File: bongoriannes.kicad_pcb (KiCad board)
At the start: 2 copper layers, 100 x 80 mm, 74 parts, among them J1 VRAM, J10 VIDEO, J11 PPU21, J13 SOUND, J14 POWER, J2 CART_FRONT, J3 CART_BOTTOM, J4 CPU_RP2A03, J5 PRG_WRAM, J7 PPU, P1 P1, P2 P2, Q1 2SC2021, Q2 2SC2021, Q3 2SA937, SW1 SW_Push, U1 74LS373, U2 74LS139, U3 74LS368, U4 74LS368, Y1 21.47727

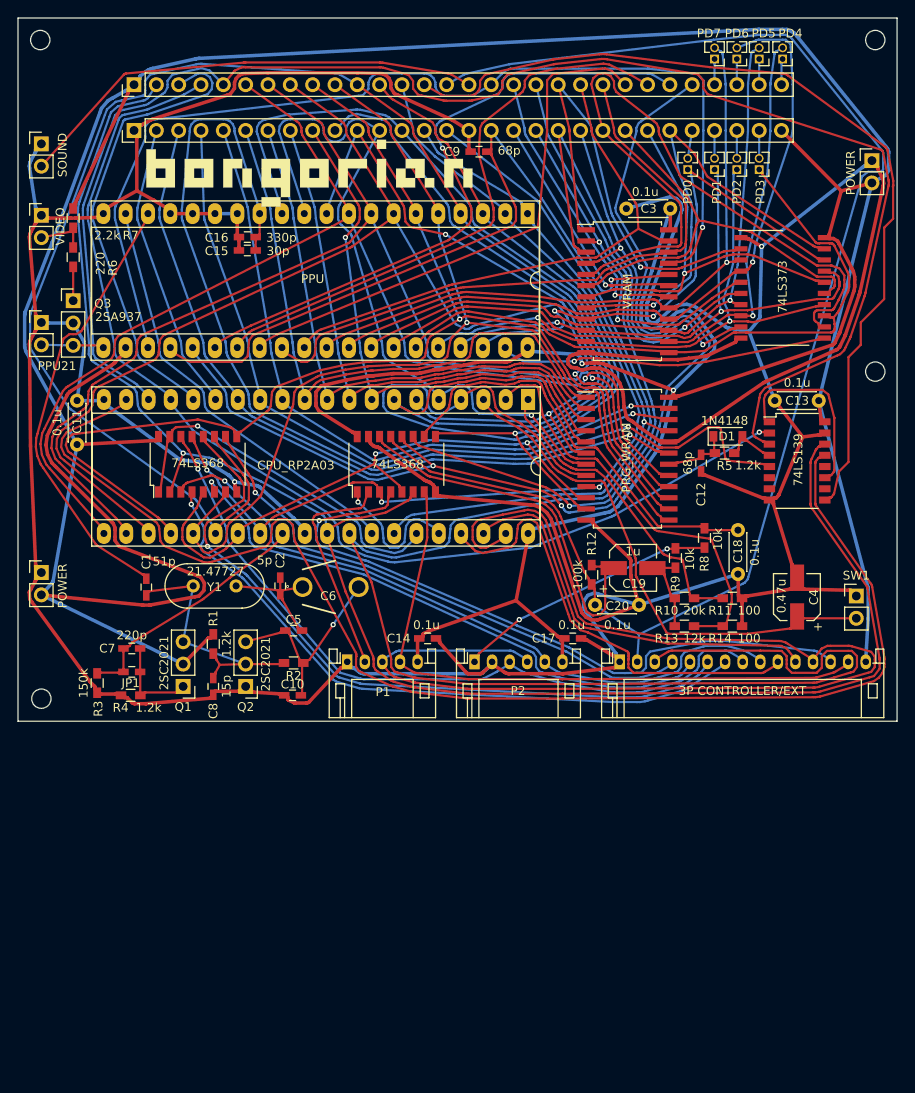
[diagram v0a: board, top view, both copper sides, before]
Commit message: meishi_size
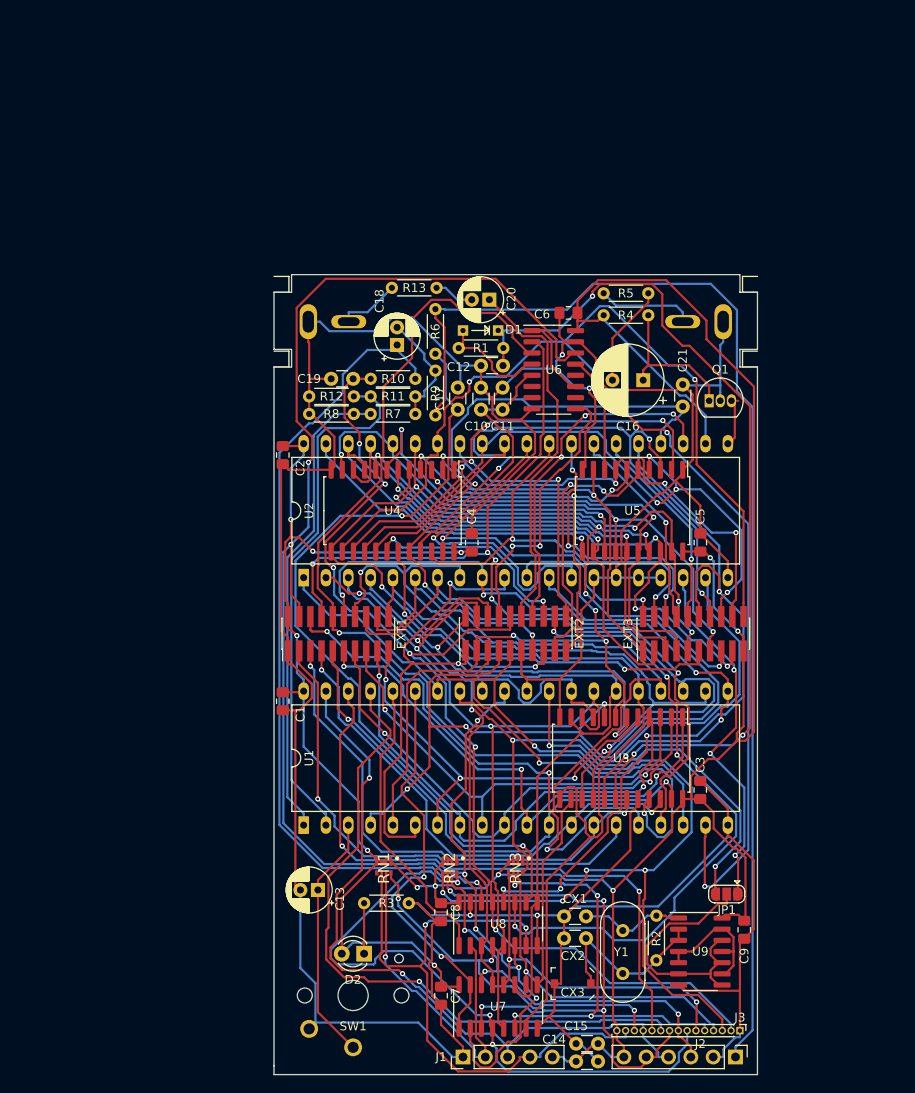
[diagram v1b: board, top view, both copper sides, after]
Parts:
- removed 3P CONTROLLER/EXT: EXT, Connectors_JST:JST_PH_S15B-PH-K_15x2.00mm_Angled
- removed G*** (x2): LOGO, GAME:bongorian
- removed G***: LOGO, GAME:fami
- removed J10: VIDEO, Pin_Headers:Pin_Header_Straight_1x02_Pitch2.54mm
- removed J11: PPU21, Pin_Headers:Pin_Header_Straight_1x02_Pitch2.54mm
- removed J13: SOUND, Pin_Headers:Pin_Header_Straight_1x02_Pitch2.54mm
- removed J14: POWER, Pin_Headers:Pin_Header_Straight_1x02_Pitch2.54mm
- removed J7: PPU, Housings_DIP:DIP-40_W15.24mm_Socket_LongPads
- removed JP15: PD0, Pin_Headers:Pin_Header_Straight_1x02_Pitch1.27mm
- removed JP17: PD1, Pin_Headers:Pin_Header_Straight_1x02_Pitch1.27mm
- removed JP18: PD7, Pin_Headers:Pin_Header_Straight_1x02_Pitch1.27mm
- removed JP19: PD2, Pin_Headers:Pin_Header_Straight_1x02_Pitch1.27mm
- removed JP20: PD6, Pin_Headers:Pin_Header_Straight_1x02_Pitch1.27mm
- removed JP21: PD3, Pin_Headers:Pin_Header_Straight_1x02_Pitch1.27mm
- removed JP22: PD5, Pin_Headers:Pin_Header_Straight_1x02_Pitch1.27mm
- removed JP23: PD4, Pin_Headers:Pin_Header_Straight_1x02_Pitch1.27mm
- removed P1: P1, Connectors_JST:JST_PH_S5B-PH-K_05x2.00mm_Angled
- removed P2: P2, Connectors_JST:JST_PH_S6B-PH-K_06x2.00mm_Angled
- removed POWER: Conn_01x02, Pin_Headers:Pin_Header_Straight_1x02_Pitch2.54mm
- removed Q2: 2SC2021, Pin_Headers:Pin_Header_Straight_1x03_Pitch2.54mm
- removed Q3: 2SA937, Pin_Headers:Pin_Header_Straight_1x03_Pitch2.54mm
- removed R14: 100, Resistors_SMD:R_0603_HandSoldering
- removed hole1, hole2, hole3, hole4: MountingHole_2.2mm_M2, Mounting_Holes:MountingHole_2.2mm_M2
- added C21: 68p, Capacitor_THT:C_Disc_D3.0mm_W1.6mm_P2.50mm, F.Cu at (146.5, 85.0)
- added CX1: 22p, Capacitor_THT:C_Disc_D3.0mm_W1.6mm_P2.50mm, F.Cu at (135.5, 143.0)
- added CX2: 15p, Capacitor_THT:C_Disc_D3.0mm_W1.6mm_P2.50mm, F.Cu at (135.5, 145.5)
- added CX3: CTRIM, Capacitor_SMD:C_Trimmer_Murata_TZC3, F.Cu at (134.0, 150.7)
- added D2: LED, LED_THT:LED_D3.0mm, F.Cu at (110.2, 147.2)
- added EXT1: 1-10, Connector_PinHeader_1.27mm:PinHeader_2x10_P1.27mm_Vertical_SMD, F.Cu at (107.3, 110.8)
- added EXT2: 11-20, Connector_PinHeader_1.27mm:PinHeader_2x10_P1.27mm_Vertical_SMD, F.Cu at (127.5, 110.8)
- added EXT3: 21-30, Connector_PinHeader_1.27mm:PinHeader_2x10_P1.27mm_Vertical_SMD, F.Cu at (147.7, 110.8)
- added RN1: MNR04MRAPJ103, bongorian:RESCAX50P100X200X36-8N, F.Cu at (112.5, 137.5)
- added RN2: MNR04MRAPJ103, bongorian:RESCAX50P100X200X36-8N, F.Cu at (120.0, 137.5)
- added RN3: MNR04MRAPJ103, bongorian:RESCAX50P100X200X36-8N, F.Cu at (127.5, 137.5)
- added U5: 74LS373, Package_SO:SOIC-20W_7.5x12.8mm_P1.27mm, F.Cu at (140.8, 96.8)
- added U6: 74LS139, Package_SO:SOIC-16_3.9x9.9mm_P1.27mm, F.Cu at (131.8, 80.8)
- added U7: 74LS368, Package_SO:SOIC-16_3.9x9.9mm_P1.27mm, F.Cu at (125.5, 153.2)
- added U8: 74LS368, Package_SO:SOIC-16_3.9x9.9mm_P1.27mm, F.Cu at (125.5, 143.9)
- added U9: 74HC04, Package_SO:SOIC-14_3.9x8.7mm_P1.27mm, F.Cu at (148.5, 147.0)
- C1: value 51p -> 0.1u; footprint Capacitors_SMD:C_0603_HandSoldering -> Capacitor_SMD:C_0805_2012Metric_Pad1.15x1.40mm_HandSolder
- C10: value 51p -> 330p; footprint Capacitors_SMD:C_0603_HandSoldering -> Capacitor_THT:C_Disc_D3.0mm_W1.6mm_P2.50mm
- C11: value 0.1u -> 30p; footprint Capacitors_THT:C_Disc_D4.3mm_W1.9mm_P5.00mm -> Capacitor_THT:C_Disc_D3.0mm_W1.6mm_P2.50mm
- C12, C14, C17: footprint Capacitors_SMD:C_0603_HandSoldering -> Capacitor_THT:C_Disc_D3.0mm_W1.6mm_P2.50mm
- C13: value 0.1u -> 0.47u; footprint Capacitors_THT:C_Disc_D4.3mm_W1.9mm_P5.00mm -> Capacitor_THT:CP_Radial_D5.0mm_P2.00mm
- C15: value 30p -> 0.1u; footprint Capacitors_SMD:C_0603_HandSoldering -> Capacitor_THT:C_Disc_D3.0mm_W1.6mm_P2.50mm
- C16: value 330p -> 220u; footprint Capacitors_SMD:C_0603_HandSoldering -> Capacitor_THT:CP_Radial_D8.0mm_P3.50mm
- C18: value 0.1u -> 1u; footprint Capacitors_THT:C_Disc_D4.3mm_W1.9mm_P5.00mm -> Capacitor_THT:CP_Radial_D5.0mm_P2.00mm
- C19: value 1u -> 0.1u; footprint Capacitors_SMD:CP_Elec_5x5.3 -> Capacitor_THT:C_Disc_D3.0mm_W1.6mm_P2.50mm
- C2: value 5p -> 0.1u; footprint Capacitors_SMD:C_0603_HandSoldering -> Capacitor_SMD:C_0805_2012Metric_Pad1.15x1.40mm_HandSolder
- C20: value 0.1u -> 4.7u; footprint Capacitors_THT:C_Disc_D4.3mm_W1.9mm_P5.00mm -> Capacitor_THT:CP_Radial_D5.0mm_P2.00mm
- C3: footprint Capacitors_THT:C_Disc_D4.3mm_W1.9mm_P5.00mm -> Capacitor_SMD:C_0805_2012Metric_Pad1.15x1.40mm_HandSolder
- C4: value 0.47u -> 0.1u; footprint Capacitors_SMD:CP_Elec_5x5.3 -> Capacitor_SMD:C_0805_2012Metric_Pad1.15x1.40mm_HandSolder
- C5: value 18p -> 0.1u; footprint Capacitors_SMD:C_0603_HandSoldering -> Capacitor_SMD:C_0805_2012Metric_Pad1.15x1.40mm_HandSolder
- C6: value 30p -> 0.1u; footprint SamacSys_Parts:TZ03(B) -> Capacitor_SMD:C_0805_2012Metric_Pad1.15x1.40mm_HandSolder
- C7: value 220p -> 0.1u; footprint Capacitors_SMD:C_0603_HandSoldering -> Capacitor_SMD:C_0805_2012Metric_Pad1.15x1.40mm_HandSolder
- C8: value 15p -> 0.1u; footprint Capacitors_SMD:C_0603_HandSoldering -> Capacitor_SMD:C_0805_2012Metric_Pad1.15x1.40mm_HandSolder
- C9: value 68p -> 0.1u; footprint Capacitors_SMD:C_0603_HandSoldering -> Capacitor_SMD:C_0805_2012Metric_Pad1.15x1.40mm_HandSolder
- D1: value 1N4148 -> 1S953; footprint Diodes_SMD:D_SOD-123 -> bongorian:DIODE_SHORT
- J1: value VRAM -> P1; footprint Housings_SOIC:SOIC-24W_7.5x15.4mm_Pitch1.27mm -> Connector_PinHeader_2.54mm:PinHeader_1x05_P2.54mm_Vertical
- J2: value CART_FRONT -> P2; footprint Pin_Headers:Pin_Header_Straight_1x30_Pitch2.54mm -> Connector_PinHeader_2.54mm:PinHeader_1x06_P2.54mm_Vertical
- J3: value CART_BOTTOM -> P3; footprint Pin_Headers:Pin_Header_Straight_1x30_Pitch2.54mm -> Connector_PinHeader_1.00mm:PinHeader_1x15_P1.00mm_Vertical
- J4: value CPU_RP2A03 -> VIDEO; footprint Housings_DIP:DIP-40_W15.24mm_Socket_LongPads -> bongorian:RCA_RJ2410N
- J5: value PRG_WRAM -> AUDIO; footprint Housings_SOIC:SOIC-24W_7.5x15.4mm_Pitch1.27mm -> bongorian:RCA_RJ2410N
- JP1: value Jumper -> CLOCK; footprint Capacitors_SMD:C_0603_HandSoldering -> Jumper:SolderJumper-3_P1.3mm_Open_RoundedPad1.0x1.5mm
- Q1: value 2SC2021 -> 2SA1015; footprint Pin_Headers:Pin_Header_Straight_1x03_Pitch2.54mm -> Package_TO_SOT_THT:TO-92_Inline
- R1, R9: footprint Resistors_SMD:R_0603_HandSoldering -> Resistor_THT:R_Axial_DIN0204_L3.6mm_D1.6mm_P5.08mm_Horizontal
- R10: value 20k -> 100k; footprint Resistors_SMD:R_0603_HandSoldering -> Resistor_THT:R_Axial_DIN0204_L3.6mm_D1.6mm_P5.08mm_Horizontal
- R11: value 100 -> 12k; footprint Resistors_SMD:R_0603_HandSoldering -> Resistor_THT:R_Axial_DIN0204_L3.6mm_D1.6mm_P5.08mm_Horizontal
- R12: value 100k -> 100; footprint Resistors_SMD:R_0603_HandSoldering -> Resistor_THT:R_Axial_DIN0204_L3.6mm_D1.6mm_P5.08mm_Horizontal
- R13: value 12k -> 1k; footprint Resistors_SMD:R_0603_HandSoldering -> Resistor_THT:R_Axial_DIN0204_L3.6mm_D1.6mm_P5.08mm_Horizontal
- R2: value 220k -> 1M; footprint Resistors_SMD:R_0603_HandSoldering -> Resistor_THT:R_Axial_DIN0204_L3.6mm_D1.6mm_P5.08mm_Horizontal
- R3: value 150k -> R; footprint Resistors_SMD:R_0603_HandSoldering -> Resistor_THT:R_Axial_DIN0204_L3.6mm_D1.6mm_P5.08mm_Horizontal
- R4: value 1.2k -> 150; footprint Resistors_SMD:R_0603_HandSoldering -> Resistor_THT:R_Axial_DIN0204_L3.6mm_D1.6mm_P5.08mm_Horizontal
- R5: value 1.2k -> 75; footprint Resistors_SMD:R_0603_HandSoldering -> Resistor_THT:R_Axial_DIN0204_L3.6mm_D1.6mm_P5.08mm_Horizontal
- R6: value 220 -> 10k; footprint Resistors_SMD:R_0603_HandSoldering -> Resistor_THT:R_Axial_DIN0204_L3.6mm_D1.6mm_P5.08mm_Horizontal
- R7: value 2.2k -> 20k; footprint Resistors_SMD:R_0603_HandSoldering -> Resistor_THT:R_Axial_DIN0204_L3.6mm_D1.6mm_P5.08mm_Horizontal
- R8: value 10k -> 100; footprint Resistors_SMD:R_0603_HandSoldering -> Resistor_THT:R_Axial_DIN0204_L3.6mm_D1.6mm_P5.08mm_Horizontal
- SW1: footprint Pin_Headers:Pin_Header_Straight_1x02_Pitch2.54mm -> keyswitches:PG1350
- U1: value 74LS373 -> 2A03_CPU; footprint Housings_SOIC:SO-20_12.8x7.5mm_Pitch1.27mm -> bongorian:DIP-40_W15.24mm_LongPads_hoso
- U2: value 74LS139 -> 2C02_PPU; footprint Housings_SSOP:SOP-16_4.4x10.4mm_Pitch1.27mm -> bongorian:DIP-40_W15.24mm_LongPads_hoso
- U3: value 74LS368 -> SRAM; footprint Housings_SSOP:SOP-16_4.4x10.4mm_Pitch1.27mm -> Package_SO:SOIC-24W_7.5x15.4mm_P1.27mm
- U4: value 74LS368 -> VRAM; footprint Housings_SSOP:SOP-16_4.4x10.4mm_Pitch1.27mm -> Package_SO:SOIC-24W_7.5x15.4mm_P1.27mm
- Y1: value 21.47727 -> Crystal; footprint Crystals:Crystal_HC49-U_Vertical -> Crystal:Crystal_HC49-4H_Vertical
- moved J3 127.8 mm to (153.0, 156.0), turned to 270 degrees
- moved J2 125.7 mm to (152.5, 159.0), turned to 270 degrees
- moved C15 97.7 mm to (134.4, 157.5)
- moved C9 93.5 mm to (153.5, 144.5), turned to 270 degrees
- moved J1 89.1 mm to (121.5, 159.0), turned to 90 degrees
- moved C13 76.2 mm to (105.0, 140.0), turned to 180 degrees
- moved SW1 73.1 mm to (109.0, 152.0)
- moved JP1 72.2 mm to (151.5, 140.5), turned to 180 degrees
- moved R4 69.0 mm to (137.5, 74.6), turned to 0 degrees
- moved Q1 68.1 mm to (149.5, 84.3), turned to 0 degrees
- moved C3 66.7 mm to (148.5, 128.6), turned to 90 degrees
- moved Y1 62.7 mm to (139.7, 144.6), turned to 270 degrees
- moved U1 61.5 mm to (127.5, 125.0), turned to 90 degrees
- moved U3 58.6 mm to (139.5, 125.0), turned to 270 degrees
- moved R2 53.4 mm to (143.5, 148.0), turned to 90 degrees
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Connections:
- C1 pad 1: PPU_CLK -> VCC
- C1 pad 2: Net-(C1-Pad2) -> GND
- C10 pad 1: GND -> /DBE#
- C10 pad 2: Net-(C10-Pad2) -> GND
- C11 pad 1: GND -> /DBE#
- C11 pad 2: VCC -> GND
- C13 pad 1: GND -> /RES#$%
- C13 pad 2: VCC -> GND
- C14 pad 1: VCC -> GND
- C14 pad 2: GND -> VCC
- C15 pad 2: DBE# -> VCC
- C16 pad 1: GND -> Net-(C16-Pad1)
- C16 pad 2: DBE# -> Net-(C16-Pad2)
- C17 pad 1: VCC -> /MIC_IN'
- C18 pad 1: MICIN' -> /SOUND_I'
- C18 pad 2: GND -> Net-(C18-Pad2)
- C19 pad 1: SOUNDI' -> /SOUND_I
- C19 pad 2: Net-(C19-Pad2) -> GND
- C2 pad 1: Net-(C2-Pad1) -> VCC
- C2 pad 2: Net-(C2-Pad1) -> GND
- C20 pad 1: SOUNDI -> /SOUND_OUT
- C20 pad 2: GND -> Net-(C20-Pad2)
- C3 pad 1: GND -> VCC
- C3 pad 2: VCC -> GND
- C4 pad 1: Net-(C4-Pad1) -> VCC
- C5 pad 1: Net-(C10-Pad2) -> VCC
- C5 pad 2: Net-(C2-Pad1) -> GND
- C6 pad 1: Net-(C2-Pad1) -> VCC
- C6 pad 2: Net-(C10-Pad2) -> GND
- C7 pad 1: Net-(C7-Pad1) -> VCC
- C7 pad 2: CPU_CLK -> GND
- C8 pad 1: GND -> VCC
- C8 pad 2: Net-(C1-Pad2) -> GND
- C9 pad 1: RD#$% -> VCC
- D1 pad 2: RAMSEL# -> /RAMSEL#
- J1 pad 1: PA7 -> GND
- J1 pad 2: PA6 -> /4016_D0$
- J1 pad 3: PA5 -> /OUT0
- J1 pad 4: PA4 -> /4016_CUP$
- J1 pad 5: PA3 -> VCC
- J2 pad 1: GND -> /MIC_IN
- J2 pad 2: A11 -> GND
- J2 pad 3: A10 -> /4017_D0$
- J2 pad 4: A9 -> /OUT0
- J2 pad 5: A8 -> /4017_CUP$
- J2 pad 6: A7 -> VCC
- J3 pad 1: VCC -> GND
- J3 pad 10: D3 -> /OUT2
- J3 pad 11: D2 -> /OUT1
- J3 pad 12: D1 -> /OUT0
- J3 pad 13: D0 -> /4016_D1$
- J3 pad 14: ROMSEL# -> /4016_CUP$
- J3 pad 15: SOUNDI -> VCC
- J3 pad 2: CLKOUT -> /SOUND_I
- J3 pad 3: A12 -> /IRQ#$
- J3 pad 4: A13 -> /4017_D4$
- J3 pad 5: A14 -> /4017_D3$
- J3 pad 6: D7 -> /4017_D2$
- J3 pad 7: D6 -> /4017_D1$
- J3 pad 8: D5 -> /4017_D0$
- J3 pad 9: D4 -> /4017_CUP$
- J4 pad 1: AUXA -> Net-(J4-Pad1)
- J4 pad 2: AUXB -> GND
- J5 pad 1: A7 -> Net-(J5-Pad1)
- J5 pad 2: A6 -> GND
- JP1 pad 1: CPU_CLK -> /PPU_CLK
- JP1 pad 2: Net-(C7-Pad1) -> Net-(JP1-Pad2)
- Q1 pad 1: Net-(C7-Pad1) -> Net-(C16-Pad1)
- Q1 pad 2: VCC -> GND
- Q1 pad 3: Net-(C1-Pad2) -> /VIDEO_OUT
- R1 pad 1: VCC -> /RAMSEL#
- R1 pad 2: Net-(C1-Pad2) -> Net-(C12-Pad1)
- R10 pad 1: AUXA -> /SOUND_I'
- R10 pad 2: Net-(C19-Pad2) -> /SOUND_I
- R11 pad 1: GND -> /AUX_B
- R11 pad 2: AUXA -> Net-(C18-Pad2)
- R12 pad 1: SOUNDI' -> GND
- R12 pad 2: SOUNDI -> /AUX_B
- R13 pad 1: AUXB -> Net-(J5-Pad1)
- R13 pad 2: Net-(C19-Pad2) -> Net-(C20-Pad2)
- R2 pad 1: Net-(C10-Pad2) -> Net-(CX2-Pad1)
- R2 pad 2: Net-(C1-Pad2) -> Net-(CX1-Pad1)
- R3 pad 1: CPU_CLK -> Net-(D2-Pad1)
- R4 pad 1: Net-(C7-Pad1) -> VCC
- R4 pad 2: GND -> Net-(C16-Pad1)
- R5 pad 1: RAMSEL# -> Net-(J4-Pad1)
- R5 pad 2: Net-(C12-Pad1) -> Net-(C16-Pad2)
- R6 pad 1: VIDEO -> /MIC_IN'
- R6 pad 2: Net-(Q3-Pad1) -> /MIC_IN
- R7 pad 1: VIDEO -> /AUX_A
- R7 pad 2: VCC -> Net-(C18-Pad2)
- R8 pad 1: MICIN' -> GND
- R8 pad 2: MICIN -> /AUX_A
- R9 pad 1: MICIN -> /MIC_IN
- R9 pad 2: Net-(C19-Pad2) -> Net-(C18-Pad2)
- SW1 pad 1: GND -> /RES#$%
- SW1 pad 2: Net-(C4-Pad1) -> GND
- U1 pad 1: GND -> /AUX_A
- U1 pad 10: GND -> /A6
- U1 pad 11: ALE$% -> /A7
- U1 pad 12: PA3 -> /A8
- U1 pad 13: PD3 -> /A9
- U1 pad 14: PD2 -> /A10
- U1 pad 15: PA2 -> /A11
- U1 pad 16: PA1 -> /A12
- U1 pad 17: PD1 -> /A13
- U1 pad 18: PD0 -> /A14
- U1 pad 19: PA0 -> /A15
- U1 pad 2: PA7 -> /AUX_B
- U1 pad 20: VCC -> GND
- U1 pad 3: PD7 -> /RES#$%
- U1 pad 4: PD6 -> /A0
- U1 pad 5: PA6 -> /A1
- U1 pad 6: PA5 -> /A2
- U1 pad 7: PD5 -> /A3
- U1 pad 8: PD4 -> /A4
- U1 pad 9: PA4 -> /A5
- U2 pad 1: Net-(U2-Pad1) -> /R_W#
- U2 pad 10: (no net) -> /A2
- U2 pad 11: Net-(U2-Pad1) -> /A1
- U2 pad 12: (no net) -> /A0
- U2 pad 13: A15 -> /DBE#
- U2 pad 14: CLKOUT -> GND
- U2 pad 16: VCC -> GND
- U2 pad 2: A13 -> /D0
- U2 pad 3: A14 -> /D1
- U2 pad 4: RAMSEL# -> /D2
- U2 pad 5: DBE# -> /D3
- U2 pad 6: (no net) -> /D4
- U2 pad 7: (no net) -> /D5
- U2 pad 8: GND -> /D6
- U2 pad 9: ROMSEL# -> /D7
- U3 pad 1: INP1# -> /A7
- U3 pad 10: 4017D4$ -> /D1
- U3 pad 11: D2 -> /D2
- U3 pad 12: 4017D2$ -> GND
- U3 pad 13: D0 -> /D3
- U3 pad 14: 4017D0$ -> /D4
- U3 pad 15: INP1# -> /D5
- U3 pad 16: VCC -> /D6
- U3 pad 2: CLKOUT -> /A6
- U3 pad 3: 4017CUP$ -> /A5
- U3 pad 4: 4017D1$ -> /A4
- U3 pad 5: D1 -> /A3
- U3 pad 6: 4017D3$ -> /A2
- U3 pad 7: D3 -> /A1
- U3 pad 8: GND -> /A0
- U3 pad 9: D4 -> /D0
- U4 pad 1: INP0# -> /PA7
- U4 pad 10: MICIN' -> /PD1
- U4 pad 11: PA13' -> /PD2
- U4 pad 12: PA13$% -> GND
- U4 pad 13: SOUNDI -> /PD3
- U4 pad 14: SOUNDI' -> /PD4
- U4 pad 15: GND -> /PD5
- U4 pad 16: VCC -> /PD6
- U4 pad 2: 4016D0$ -> /PA6
- U4 pad 3: D0 -> /PA5
- U4 pad 4: 4016D1$ -> /PA4
- U4 pad 5: D1 -> /PA3
- U4 pad 6: CLKOUT -> /PA2
- U4 pad 7: 4016CUP$ -> /PA1
- U4 pad 8: GND -> /PA0
- U4 pad 9: D2 -> /PD0
- Y1 pad 1: Net-(C1-Pad2) -> Net-(CX1-Pad1)
- Y1 pad 2: Net-(C2-Pad1) -> Net-(CX2-Pad1)
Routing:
- net /CLKOUT: track 0.00 -> 192.8 mm, vias 0 -> 7
- net CLKOUT: track 190.2 -> 0.00 mm, vias 1 -> 0
- net D2: track 184.3 -> 0.00 mm, vias 1 -> 0
- net IRQ#$: track 182.9 -> 0.00 mm
- net A14: track 174.9 -> 0.00 mm
- net VCC: track 527.5 -> 352.8 mm, vias 2 -> 12
- net SOUNDI: track 165.2 -> 0.00 mm
- net A15: track 151.2 -> 0.00 mm
- net OUT0: track 139.8 -> 0.00 mm
- net D5: track 138.7 -> 0.00 mm, vias 1 -> 0
- net D4: track 137.0 -> 0.00 mm, vias 1 -> 0
- net /MIC_IN: track 0.00 -> 136.3 mm
- net D6: track 134.1 -> 0.00 mm, vias 1 -> 0
- net D7: track 134.1 -> 0.00 mm, vias 1 -> 0
- net A0: track 129.2 -> 0.00 mm
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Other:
- board size 100 x 80 mm -> 55 x 91 mm
- net class POWER: trace_width 0.4 -> 0.25
- board text removed: "FAMICOM CLONE TEST BOARD rev.1 20180628"
